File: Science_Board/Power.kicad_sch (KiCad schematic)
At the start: 48 parts, among them IC1 TCKE603RA, IC2 TCKE603RA, IC3 TCKE603RM, J21 Molex_Megafit_02, J3 Molex_Megafit_02, J4 Molex_Megafit_02, Q1 BS250, Q2 NMOS, Q3 NMOS, Q4 NMOS, U1 AP63205WU

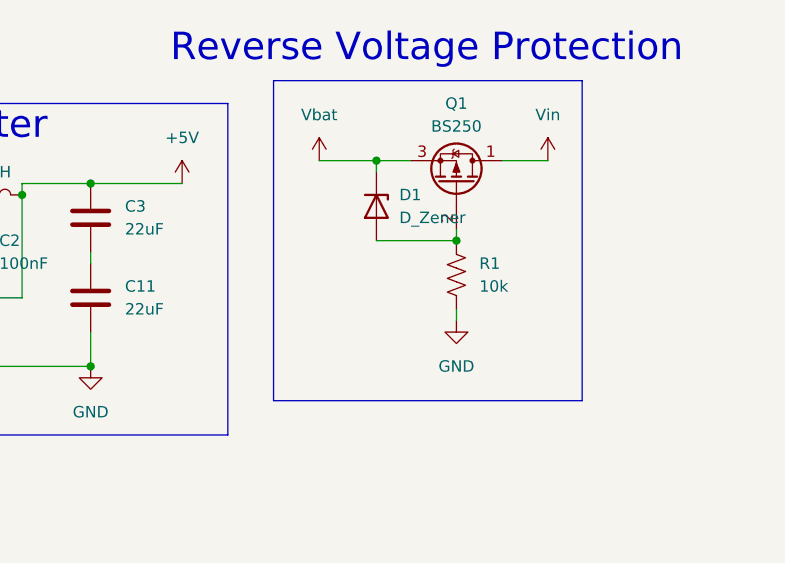
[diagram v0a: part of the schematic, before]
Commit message: created decoupling capacitors
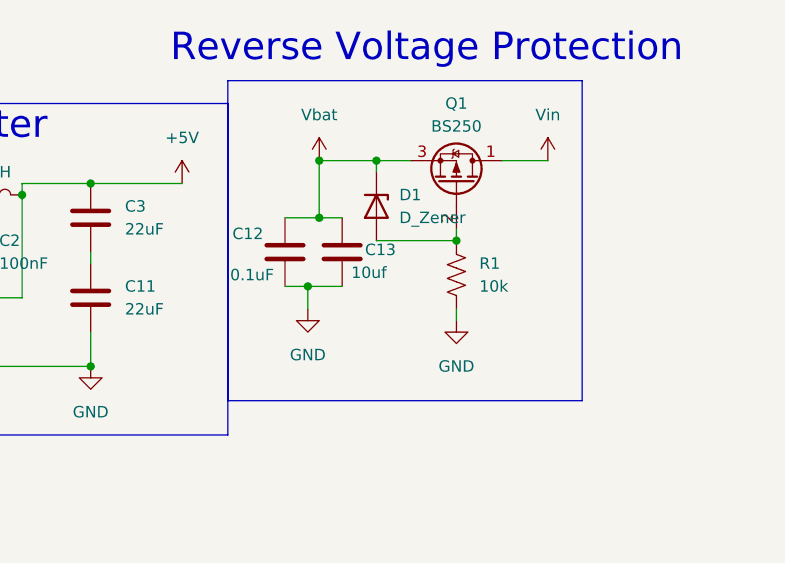
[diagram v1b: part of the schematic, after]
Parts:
- added C12: 0.1uF, symbol Device:C
- added C13: 10uf, symbol Device:C
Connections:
- net GND: now also C12.2, C13.1
- net Vbat: now also C12.1, C13.2
